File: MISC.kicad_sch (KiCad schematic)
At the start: 16 parts

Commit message: workday
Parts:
- D10, D11, D12, D13, D14, D15, D8, D9: footprint LED_SMD:LED_WS2812B-2020_PLCC4_2.0x2.0mm -> UTSVT_Passive:WS2812B-2020
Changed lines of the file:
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@@
 			)
 		)
-		(property "Footprint" "LED_SMD:LED_WS2812B-2020_PLCC4_2.0x2.0mm"
+		(property "Footprint" "UTSVT_Passive:WS2812B-2020"
 			(at 103.505 46.99 0)
 			(effects
@@
 			)
 		)
-		(property "Footprint" "LED_SMD:LED_WS2812B-2020_PLCC4_2.0x2.0mm"
+		(property "Footprint" "UTSVT_Passive:WS2812B-2020"
 			(at 122.555 46.99 0)
 			(effects
@@
 			)
 		)
-		(property "Footprint" "LED_SMD:LED_WS2812B-2020_PLCC4_2.0x2.0mm"
+		(property "Footprint" "UTSVT_Passive:WS2812B-2020"
 			(at 180.34 46.99 0)
 			(effects
@@
 			)
 		)
-		(property "Footprint" "LED_SMD:LED_WS2812B-2020_PLCC4_2.0x2.0mm"
+		(property "Footprint" "UTSVT_Passive:WS2812B-2020"
 			(at 45.72 46.99 0)
 			(effects
@@
 			)
 		)
-		(property "Footprint" "LED_SMD:LED_WS2812B-2020_PLCC4_2.0x2.0mm"
+		(property "Footprint" "UTSVT_Passive:WS2812B-2020"
 			(at 83.82 46.99 0)
 			(effects
@@
 			)
 		)
-		(property "Footprint" "LED_SMD:LED_WS2812B-2020_PLCC4_2.0x2.0mm"
+		(property "Footprint" "UTSVT_Passive:WS2812B-2020"
 			(at 141.605 46.99 0)
 			(effects
@@
 			)
 		)
-		(property "Footprint" "LED_SMD:LED_WS2812B-2020_PLCC4_2.0x2.0mm"
+		(property "Footprint" "UTSVT_Passive:WS2812B-2020"
 			(at 64.77 46.99 0)
 			(effects
@@
 			)
 		)
-		(property "Footprint" "LED_SMD:LED_WS2812B-2020_PLCC4_2.0x2.0mm"
+		(property "Footprint" "UTSVT_Passive:WS2812B-2020"
 			(at 160.655 46.99 0)
 			(effects

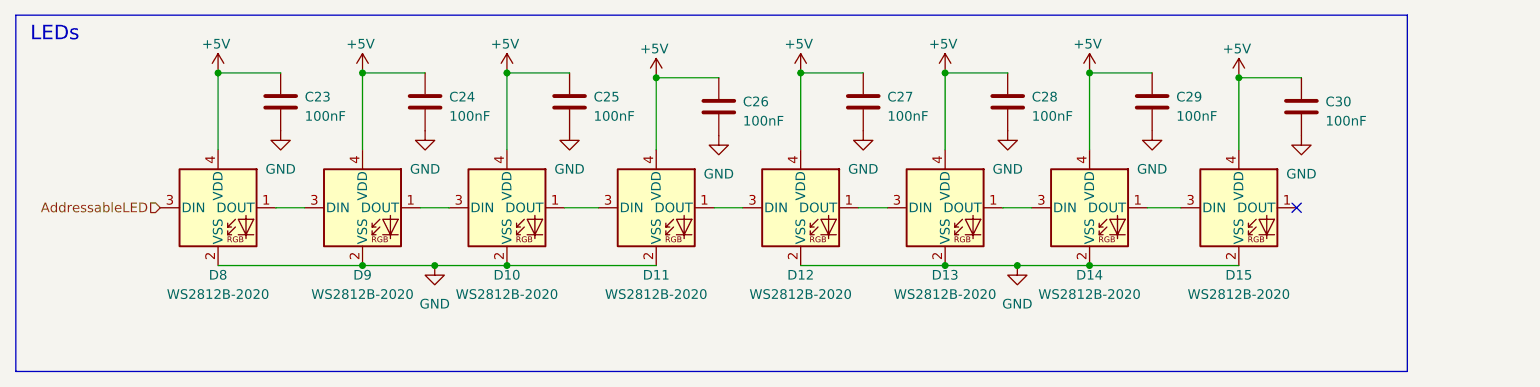
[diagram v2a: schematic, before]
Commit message: bom
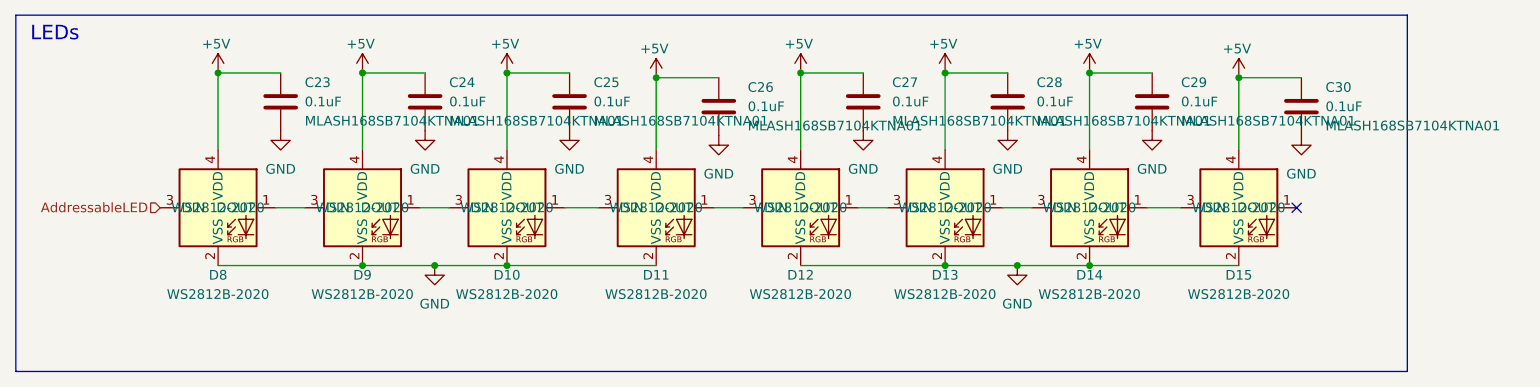
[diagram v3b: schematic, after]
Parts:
- C23, C24, C25, C26, C27, C28, C29, C30: value 100nF -> 0.1uF; Mouser Part Number (none) -> MLASH168SB7104KTNA01
- D10, D11, D12, D13, D14, D15, D8, D9: Mouser Part Number (none) -> WS2812-2020
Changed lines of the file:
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@@
 			)
 		)
+		(property "Mouser Part Number" "WS2812-2020"
+			(at 102.235 39.37 0)
+			(effects
+				(font
+					(size 1.27 1.27)
+				)
+			)
+		)
 		(pin "3"
 		)
@@
 		(fields_autoplaced yes)
 		(property "Reference" "C28"
-			(at 151.765 24.765 0)
+			(at 152.4 22.8599 0)
 			(effects
 				(font
@@
 			)
 		)
-		(property "Value" "100nF"
-			(at 151.765 27.305 0)
+		(property "Value" "0.1uF"
+			(at 152.4 25.3999 0)
 			(effects
 				(font
@@
 			)
 		)
+		(property "Mouser Part Number" "MLASH168SB7104KTNA01"
+			(at 152.4 27.9399 0)
+			(effects
+				(font
+					(size 1.27 1.27)
+				)
+				(justify left)
+			)
+		)
 		(pin "1"
 		)
@@
 			)
 		)
+		(property "Mouser Part Number" "WS2812-2020"
+			(at 121.285 39.37 0)
+			(effects
+				(font
+					(size 1.27 1.27)
+				)
+			)
+		)
 		(pin "3"
 		)
@@
 			)
 		)
+		(property "Mouser Part Number" "WS2812-2020"
+			(at 179.07 39.37 0)
+			(effects
+				(font
+					(size 1.27 1.27)
+				)
+			)
+		)
 		(pin "3"
 		)
@@
 			)
 		)
+		(property "Mouser Part Number" "WS2812-2020"
+			(at 44.45 39.37 0)
+			(effects
+				(font
+					(size 1.27 1.27)
+				)
+			)
+		)
 		(pin "3"
 		)
@@
 			)
 		)
+		(property "Mouser Part Number" "WS2812-2020"
+			(at 82.55 39.37 0)
+			(effects
+				(font
+					(size 1.27 1.27)
+				)
+			)
+		)
 		(pin "3"
 		)
@@
 			)
 		)
+		(property "Mouser Part Number" "WS2812-2020"
+			(at 140.335 39.37 0)
+			(effects
+				(font
+					(size 1.27 1.27)
+				)
+			)
+		)
 		(pin "3"
 		)
@@
 		(fields_autoplaced yes)
 		(property "Reference" "C26"
-			(at 113.665 25.4 0)
+			(at 114.3 23.4949 0)
 			(effects
 				(font
@@
 			)
 		)
-		(property "Value" "100nF"
-			(at 113.665 27.94 0)
+		(property "Value" "0.1uF"
+			(at 114.3 26.0349 0)
 			(effects
 				(font
@@
 			)
 		)
+		(property "Mouser Part Number" "MLASH168SB7104KTNA01"
+			(at 114.3 28.5749 0)
+			(effects
+				(font
+					(size 1.27 1.27)
+				)
+				(justify left)
+			)
+		)
 		(pin "1"
 		)
@@
 		(fields_autoplaced yes)
 		(property "Reference" "C25"
-			(at 93.98 24.765 0)
+			(at 93.98 22.8599 0)
 			(effects
 				(font
@@
 			)
 		)
-		(property "Value" "100nF"
-			(at 93.98 27.305 0)
+		(property "Value" "0.1uF"
+			(at 93.98 25.3999 0)
 			(effects
 				(font
@@
 			)
 		)
+		(property "Mouser Part Number" "MLASH168SB7104KTNA01"
+			(at 93.98 27.9399 0)
+			(effects
+				(font
+					(size 1.27 1.27)
+				)
+				(justify left)
+			)
+		)
 		(pin "1"
 		)
@@
 		(fields_autoplaced yes)
 		(property "Reference" "C29"
-			(at 170.815 24.765 0)
+			(at 171.45 22.8599 0)
 			(effects
 				(font
@@
 			)
 		)
-		(property "Value" "100nF"
-			(at 170.815 27.305 0)
+		(property "Value" "0.1uF"
+			(at 171.45 25.3999 0)
 			(effects
 				(font
@@
 			)
 		)
+		(property "Mouser Part Number" "MLASH168SB7104KTNA01"
+			(at 171.45 27.9399 0)
+			(effects
+				(font
+					(size 1.27 1.27)
+				)
+				(justify left)
+			)
+		)
 		(pin "1"
 		)
@@
 			)
 		)
+		(property "Mouser Part Number" "WS2812-2020"
+			(at 63.5 39.37 0)
+			(effects
+				(font
+					(size 1.27 1.27)
+				)
+			)
+		)
 		(pin "3"
 		)
@@
 		(fields_autoplaced yes)
 		(property "Reference" "C27"
-			(at 132.715 24.765 0)
+			(at 133.35 22.8599 0)
 			(effects
 				(font
@@
 			)
 		)
-		(property "Value" "100nF"
-			(at 132.715 27.305 0)
+		(property "Value" "0.1uF"
+			(at 133.35 25.3999 0)
 			(effects
 				(font
@@
 			)
 		)
+		(property "Mouser Part Number" "MLASH168SB7104KTNA01"
+			(at 133.35 27.9399 0)
+			(effects
+				(font
+					(size 1.27 1.27)
+				)
+				(justify left)
+			)
+		)
 		(pin "1"
 		)
@@
 		(fields_autoplaced yes)
 		(property "Reference" "C30"
-			(at 190.5 25.4 0)
+			(at 190.5 23.4949 0)
 			(effects
 				(font
@@
 			)
 		)
-		(property "Value" "100nF"
-			(at 190.5 27.94 0)
+		(property "Value" "0.1uF"
+			(at 190.5 26.0349 0)
 			(effects
 				(font
@@
 			)
 		)
+		(property "Mouser Part Number" "MLASH168SB7104KTNA01"
+			(at 190.5 28.5749 0)
+			(effects
+				(font
+					(size 1.27 1.27)
+				)
+				(justify left)
+			)
+		)
 		(pin "1"
 		)
@@
 		(fields_autoplaced yes)
 		(property "Reference" "C24"
-			(at 74.93 24.765 0)
+			(at 74.93 22.8599 0)
 			(effects
 				(font
@@
 			)
 		)
-		(property "Value" "100nF"
-			(at 74.93 27.305 0)
+		(property "Value" "0.1uF"
+			(at 74.93 25.3999 0)
 			(effects
 				(font
@@
 			)
 		)
+		(property "Mouser Part Number" "MLASH168SB7104KTNA01"
+			(at 74.93 27.9399 0)
+			(effects
+				(font
+					(size 1.27 1.27)
+				)
+				(justify left)
+			)
+		)
 		(pin "1"
 		)
@@
 			)
 		)
+		(property "Mouser Part Number" "WS2812-2020"
+			(at 159.385 39.37 0)
+			(effects
+				(font
+					(size 1.27 1.27)
+				)
+			)
+		)
 		(pin "3"
 		)
@@
 		(fields_autoplaced yes)
 		(property "Reference" "C23"
-			(at 55.88 24.765 0)
+			(at 55.88 22.8599 0)
 			(effects
 				(font
@@
 			)
 		)
-		(property "Value" "100nF"
-			(at 55.88 27.305 0)
+		(property "Value" "0.1uF"
+			(at 55.88 25.3999 0)
 			(effects
 				(font
@@
 			)
 		)
+		(property "Mouser Part Number" "MLASH168SB7104KTNA01"
+			(at 55.88 27.9399 0)
+			(effects
+				(font
+					(size 1.27 1.27)
+				)
+				(justify left)
+			)
+		)
